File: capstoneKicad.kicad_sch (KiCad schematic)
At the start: 7 parts, among them J1 12-24V POWER IN, U1 N7805-1PH, U2 N7803-1PH

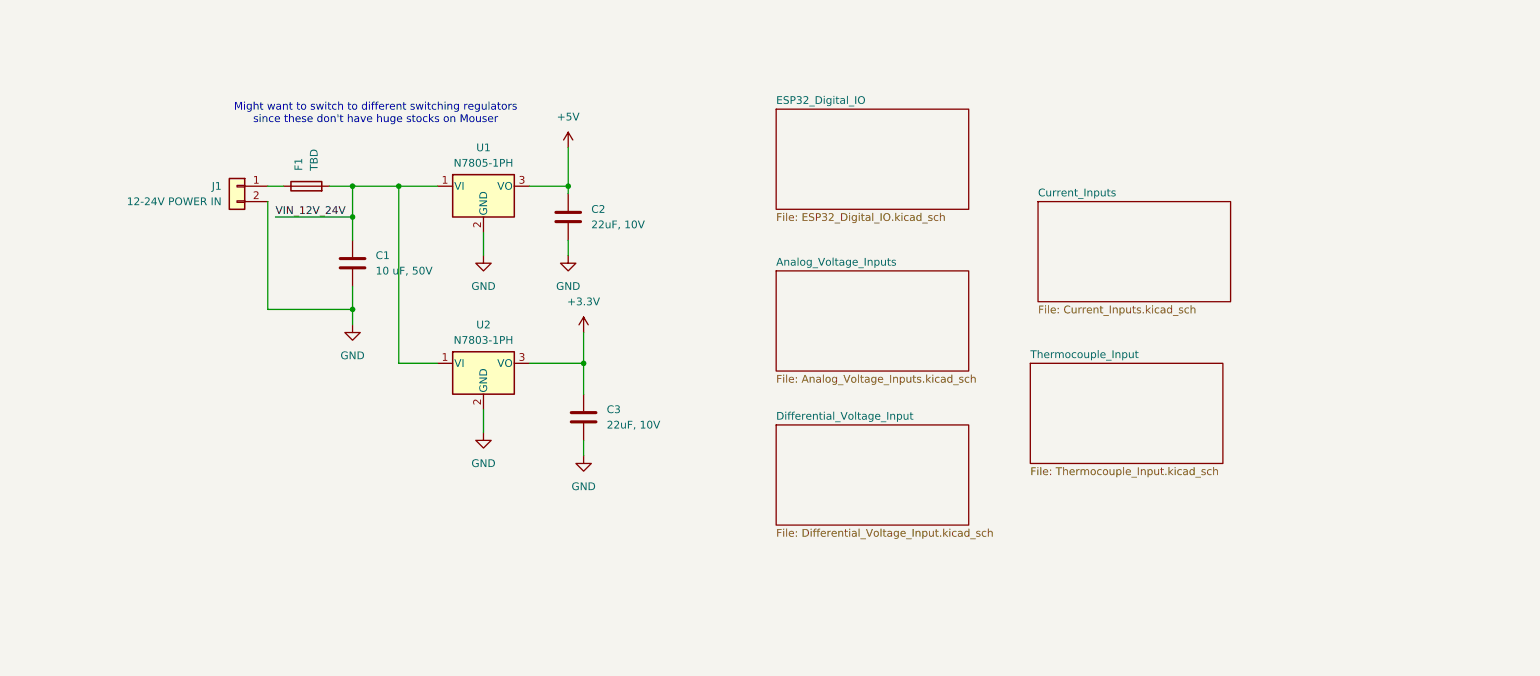
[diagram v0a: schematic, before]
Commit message: finished schematic draft 1
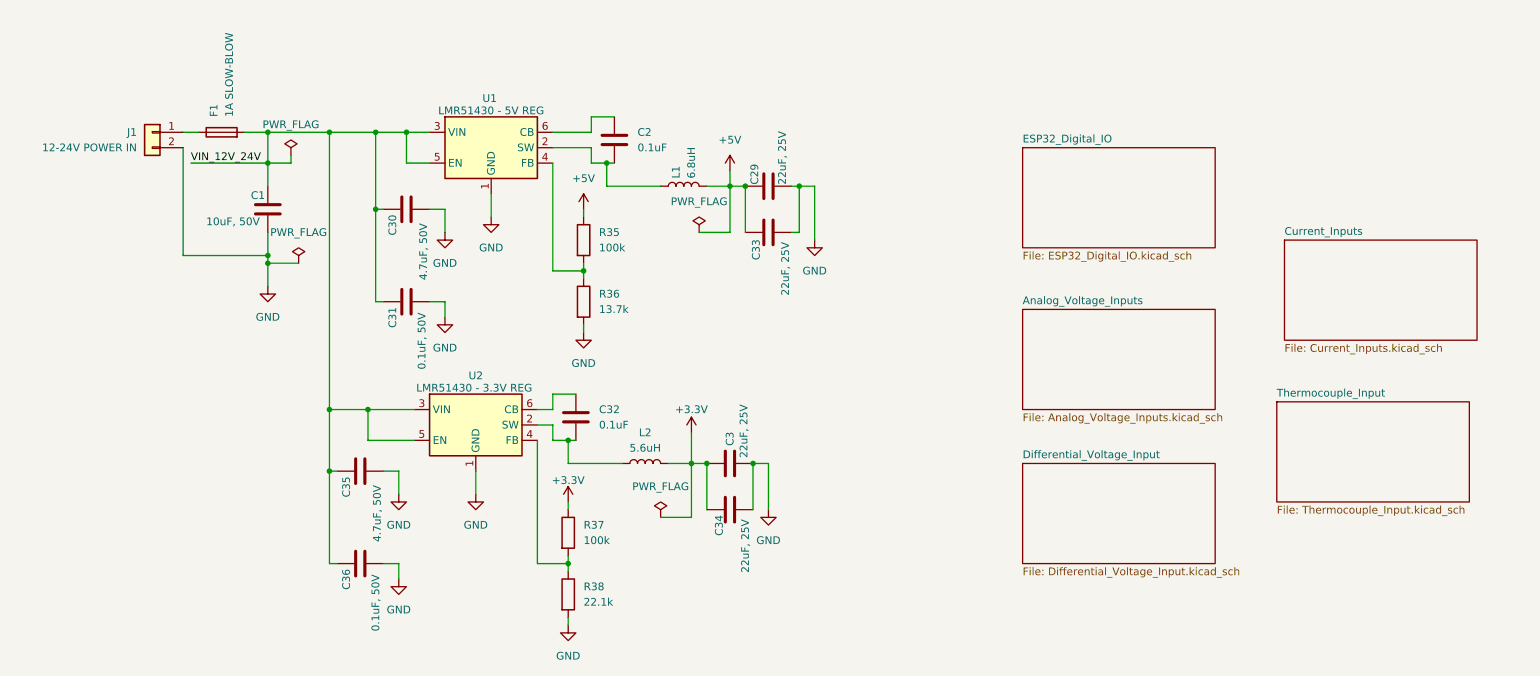
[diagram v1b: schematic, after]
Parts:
- removed U1: N7805-1PH, Package_TO_SOT_THT:TO-220-3_Vertical, symbol Regulator_Linear:LM7805_TO220
- removed U2: N7803-1PH, Package_TO_SOT_THT:TO-220-3_Vertical, symbol Regulator_Linear:LM7805_TO220
- added C29, C33, C34: 22uF, 25V, symbol Device:C
- added C30, C35: 4.7uF, 50V, symbol Device:C
- added C31, C36: 0.1uF, 50V, symbol Device:C
- added C32: 0.1uF, symbol Device:C
- added L1: 6.8uH, Package_TO_SOT_SMD:SOT-23-6, symbol Device:L
- added L2: 5.6uH, Package_TO_SOT_SMD:SOT-23-6, symbol Device:L
- added R35, R37: 100k, symbol Device:R
- added R36: 13.7k, symbol Device:R
- added R38: 22.1k, symbol Device:R
- added U1: LMR51430 - 5V REG, Package_TO_SOT_SMD:SOT-23-6, symbol Regulator_Switching:LMR51430
- added U2: LMR51430 - 3.3V REG, Package_TO_SOT_SMD:SOT-23-6, symbol Regulator_Switching:LMR51430
- C1: value 10 uF, 50V -> 10uF, 50V
- C2: value 22uF, 10V -> 0.1uF
- C3: value 22uF, 10V -> 22uF, 25V
- F1: value TBD -> 1A SLOW-BLOW; footprint (none) -> Fuse:Fuse_1206_3216Metric; MPN (none) -> 0685T1000-01; Manufacturer (none) -> Bel Fuse
- J1: footprint (none) -> TerminalBlock_Phoenix:TerminalBlock_Phoenix_MKDS-1,5-2-5.08_1x02_P5.08mm_Horizontal; MPN (none) -> 1715721; Manufacturer (none) -> Phoenix Contact
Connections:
- net +3.3V: now also C34.1, L2.2, R37.1
- net +5V: now also C29.1, C33.1, L1.2, R35.1; no longer C2.1
- net GND: now also C29.2, C30.2, C31.2, C33.2, C34.2, C35.2, C36.2, R36.2, R38.2, U1.1 (GND), U2.1 (GND); no longer C2.2
- net VIN_12V_24V: now also C30.1, C31.1, C35.1, C36.1, U1.3 (VIN), U1.5 (EN), U2.3 (VIN), U2.5 (EN)
- new net: C32.1, U2.6 (CB)
- new net: C32.2, L2.1, U2.2 (SW)
- new net: R37.2, R38.1, U2.4 (FB)
- new net: R35.2, R36.1, U1.4 (FB)
- new net: C2.2, L1.1, U1.2 (SW)
- new net: C2.1, U1.6 (CB)
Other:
- note removed: "Might want to switch to different switching regulators since these don't have huge stocks on Mouser"
- moved on the sheet: C1, C2, C3, F1, J1
